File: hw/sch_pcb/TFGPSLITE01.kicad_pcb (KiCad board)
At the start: 4 copper layers, 49.8 x 39.6 mm, 26 parts, among them IC1 CAM-M8Q, J1 SM06B-GHS-TB, J2 SM04B-GHS-TB, M1 HOLE, M2 HOLE, M3 HOLE, M4 HOLE, U1 MIC5504-3.3YM5

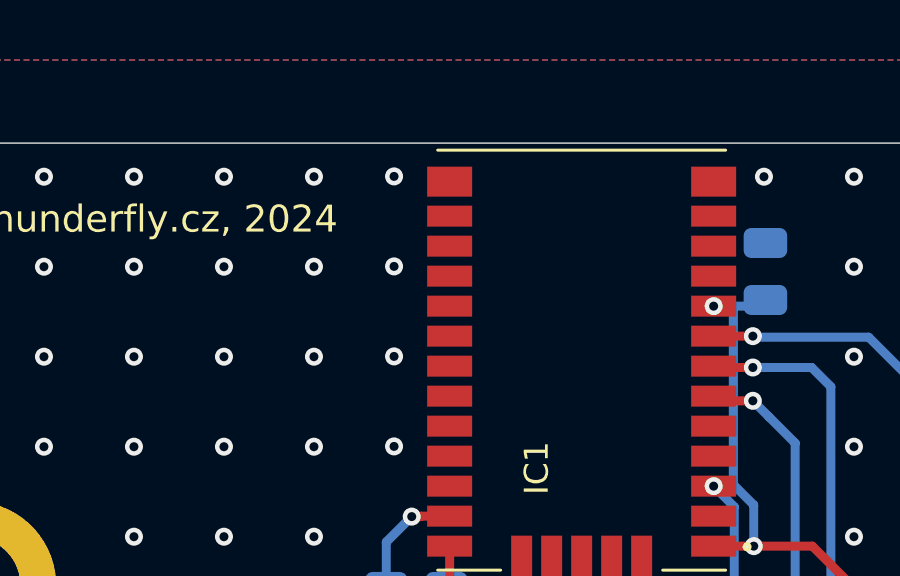
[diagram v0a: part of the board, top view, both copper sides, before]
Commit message: update actions
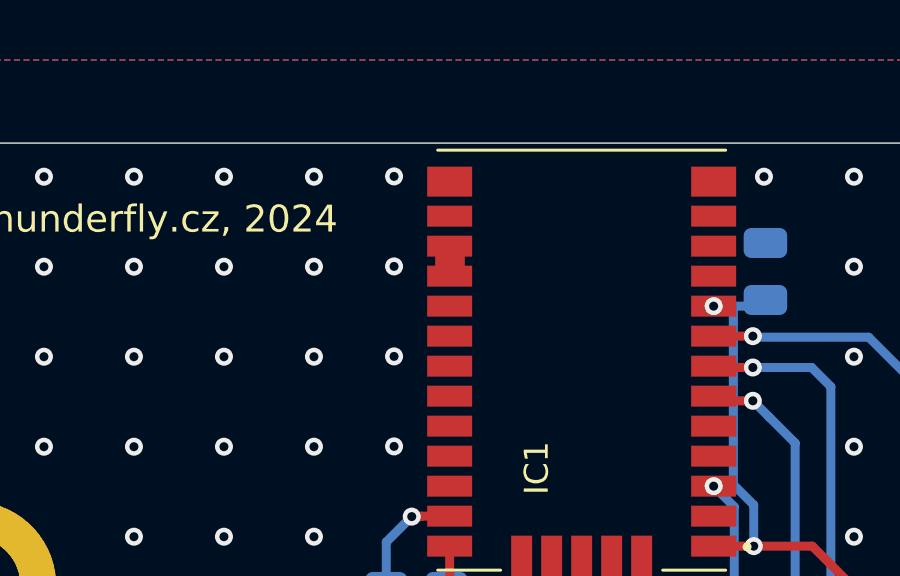
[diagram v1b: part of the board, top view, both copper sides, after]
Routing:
- net /RF: track 0.00 -> 2.00 mm
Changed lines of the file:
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@@
 		(tags "resistor")
 		(property "Reference" "R7"
-			(at 2.73 0.01 360)
+			(at 2.73 0.01 0)
 			(layer "B.SilkS")
 			(effects
@@
 		)
 		(property "Value" "R_Small"
-			(at 0 -1.65 360)
+			(at 0 -1.65 0)
 			(layer "B.Fab")
 			(effects
@@
 		)
 		(fp_text user "${REFERENCE}"
-			(at 0 0 360)
+			(at 0 0 0)
 			(layer "B.Fab")
 			(effects
@@
 		(tags "Diode SOD523")
 		(property "Reference" "D1"
-			(at 0.0025 -1.46 360)
+			(at 0.0025 -1.46 0)
 			(layer "B.SilkS")
 			(effects
@@
 		)
 		(property "Value" "BZX585-B5V6.115"
-			(at 0 -1.4 360)
+			(at 0 -1.4 0)
 			(layer "B.Fab")
 			(effects
@@
 		)
 		(fp_text user "${REFERENCE}"
-			(at 0 1.3 360)
+			(at 0 1.3 0)
 			(layer "B.Fab")
 			(effects
@@
 		(tags "capacitor")
 		(property "Reference" "C3"
-			(at 2.7575 -0.015 360)
+			(at 2.7575 -0.015 0)
 			(layer "B.SilkS")
 			(effects
@@
 		)
 		(property "Value" "100n"
-			(at 0 -1.68 360)
+			(at 0 -1.68 0)
 			(layer "B.Fab")
 			(effects
@@
 		)
 		(fp_text user "${REFERENCE}"
-			(at 0 0 360)
+			(at 0 0 0)
 			(layer "B.Fab")
 			(effects
@@
 		(tags "resistor")
 		(property "Reference" "R8"
-			(at 2.59 0.01 360)
+			(at 2.59 0.01 0)
 			(layer "B.SilkS")
 			(effects
@@
 		)
 		(property "Value" "R_Small"
-			(at 0 -1.65 360)
+			(at 0 -1.65 0)
 			(layer "B.Fab")
 			(effects
@@
 		)
 		(fp_text user "${REFERENCE}"
-			(at 0 0 360)
+			(at 0 0 0)
 			(layer "B.Fab")
 			(effects
@@
 	)
 	(segment
+		(start 131.38 89.56)
+		(end 131.38 88.56)
+		(width 0.5)
+		(layer "F.Cu")
+		(net 12)
+	)
+	(segment
+		(start 131.87 89.53)
+		(end 131.87 88.53)
+		(width 0.5)
+		(layer "F.Cu")
+		(net 12)
+	)
+	(segment
